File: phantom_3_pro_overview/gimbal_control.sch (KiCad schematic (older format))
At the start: 0 parts

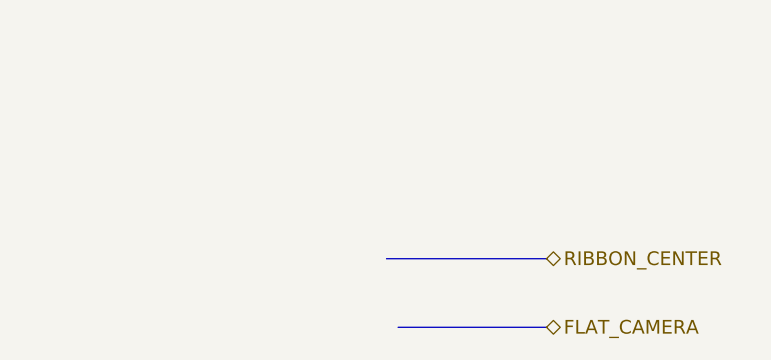
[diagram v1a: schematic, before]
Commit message: Overview: Updated gimbal control board.
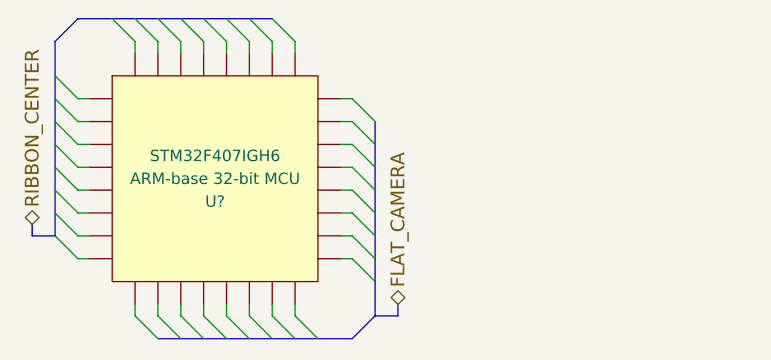
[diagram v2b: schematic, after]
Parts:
- added U?: STM32F407IGH6, ARM-base 32-bit MCU, symbol IC_PQFP32
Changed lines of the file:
@@
 EELAYER 25 0
 EELAYER END
-$Descr A4 11693 8268
+$Descr User 5118 4803
 encoding utf-8
-Sheet 9 23
+Sheet 19 23
 Title "Overview of the Phantom 3 Pro Gimbal control"
 Date ""
@@
 Comment4 ""
 $EndDescr
+Text HLabel 1650 1950 1    60   BiDi ~ 0
+RIBBON_CENTER
+Text HLabel 3250 2300 1    60   BiDi ~ 0
+FLAT_CAMERA
+$Comp
+L IC_PQFP32 U?
+U 1 1 597AFD9A
+P 2450 1750
+F 0 "U?" H 2450 1650 50  0000 C CNN
+F 1 "STM32F407IGH6" H 2450 1850 50  0000 C CNN
+F 2 "ARM-base 32-bit MCU" H 2450 1750 50  0000 C CNN
+F 3 "DOCUMENTATION" H 2450 1750 50  0001 C CNN
+	1    2450 1750
+	1    0    0    -1
+$EndComp
+Entry Wire Line
+	3050 1400 3150 1500
+Entry Wire Line
+	3050 1500 3150 1600
+Entry Wire Line
+	3050 1600 3150 1700
+Entry Wire Line
+	3050 1700 3150 1800
+Entry Wire Line
+	3050 1800 3150 1900
+Entry Wire Line
+	3050 1900 3150 2000
+Entry Wire Line
+	3050 2000 3150 2100
+Entry Wire Line
+	3050 2100 3150 2200
+Entry Wire Line
+	2100 2350 2200 2450
+Entry Wire Line
+	2200 2350 2300 2450
+Entry Wire Line
+	2300 2350 2400 2450
+Entry Wire Line
+	2400 2350 2500 2450
+Entry Wire Line
+	2500 2350 2600 2450
+Entry Wire Line
+	2600 2350 2700 2450
+Entry Wire Line
+	2700 2350 2800 2450
+Entry Wire Line
+	2800 2350 2900 2450
+Wire Wire Line
+	2100 2350 2100 2300
+Wire Wire Line
+	2200 2300 2200 2350
+Wire Wire Line
+	2300 2350 2300 2300
+Wire Wire Line
+	2400 2300 2400 2350
+Wire Wire Line
+	2500 2350 2500 2300
+Wire Wire Line
+	2600 2300 2600 2350
+Wire Wire Line
+	2700 2350 2700 2300
+Wire Wire Line
+	2800 2300 2800 2350
+Wire Wire Line
+	3000 2100 3050 2100
+Wire Wire Line
+	3050 2000 3000 2000
+Wire Wire Line
+	3000 1900 3050 1900
+Wire Wire Line
+	3050 1800 3000 1800
+Wire Wire Line
+	3000 1700 3050 1700
+Wire Wire Line
+	3050 1600 3000 1600
+Wire Wire Line
+	3000 1500 3050 1500
+Wire Wire Line
+	3050 1400 3000 1400
+Entry Bus Bus
+	3050 2450 3150 2350
 Wire Bus Line
-	3200 2100 3900 2100
+	3150 1500 3150 2350
 Wire Bus Line
-	3250 2400 3900 2400
-Text HLabel 3900 2100 2    60   BiDi ~ 0
-RIBBON_CENTER
-Text HLabel 3900 2400 2    60   BiDi ~ 0
-FLAT_CAMERA
+	2200 2450 3050 2450
+Wire Bus Line
+	3150 2350 3250 2350
+Wire Bus Line
+	3250 2350 3250 2300
+Entry Wire Line
+	1850 2100 1750 2000
+Entry Wire Line
+	1850 2000 1750 1900
+Entry Wire Line
+	1850 1900 1750 1800
+Entry Wire Line
+	1850 1800 1750 1700
+Entry Wire Line
+	1850 1700 1750 1600
+Entry Wire Line
+	1850 1600 1750 1500
+Entry Wire Line
+	1850 1500 1750 1400
+Entry Wire Line
+	1850 1400 1750 1300
+Entry Wire Line
+	2800 1150 2700 1050
+Entry Wire Line
+	2700 1150 2600 1050
+Entry Wire Line
+	2600 1150 2500 1050
+Entry Wire Line
+	2500 1150 2400 1050
+Entry Wire Line
+	2400 1150 2300 1050
+Entry Wire Line
+	2300 1150 2200 1050
+Entry Wire Line
+	2200 1150 2100 1050
+Entry Wire Line
+	2100 1150 2000 1050
+Wire Wire Line
+	2800 1150 2800 1200
+Wire Wire Line
+	2700 1200 2700 1150
+Wire Wire Line
+	2600 1150 2600 1200
+Wire Wire Line
+	2500 1200 2500 1150
+Wire Wire Line
+	2400 1150 2400 1200
+Wire Wire Line
+	2300 1200 2300 1150
+Wire Wire Line
+	2200 1150 2200 1200
+Wire Wire Line
+	2100 1200 2100 1150
+Wire Wire Line
+	1900 1400 1850 1400
+Wire Wire Line
+	1850 1500 1900 1500
+Wire Wire Line
+	1900 1600 1850 1600
+Wire Wire Line
+	1850 1700 1900 1700
+Wire Wire Line
+	1900 1800 1850 1800
+Wire Wire Line
+	1850 1900 1900 1900
+Wire Wire Line
+	1900 2000 1850 2000
+Wire Wire Line
+	1850 2100 1900 2100
+Entry Bus Bus
+	1850 1050 1750 1150
+Wire Bus Line
+	1750 2000 1750 1150
+Wire Bus Line
+	2700 1050 1850 1050
+Wire Bus Line
+	1750 2000 1650 2000
+Wire Bus Line
+	1650 2000 1650 1950
 $EndSCHEMATC
